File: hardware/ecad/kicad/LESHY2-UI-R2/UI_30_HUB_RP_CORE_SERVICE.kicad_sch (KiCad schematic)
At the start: 47 parts, among them J10 Samtec FTSH-105-01-L-DV-K-P-TR, J11 GCT USB4105-GF-A, SW20 Alps Alpine SKRTLAE010, SW21 Alps Alpine SKRTLAE010, U28 SC1512-A4, U29 Texas Instruments TPD4E05U06D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, U30 Texas Instruments TPD2EUSB30A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, U31 onsemi FSUSB42MUX, Y1 Abracon ABM8-272-T3

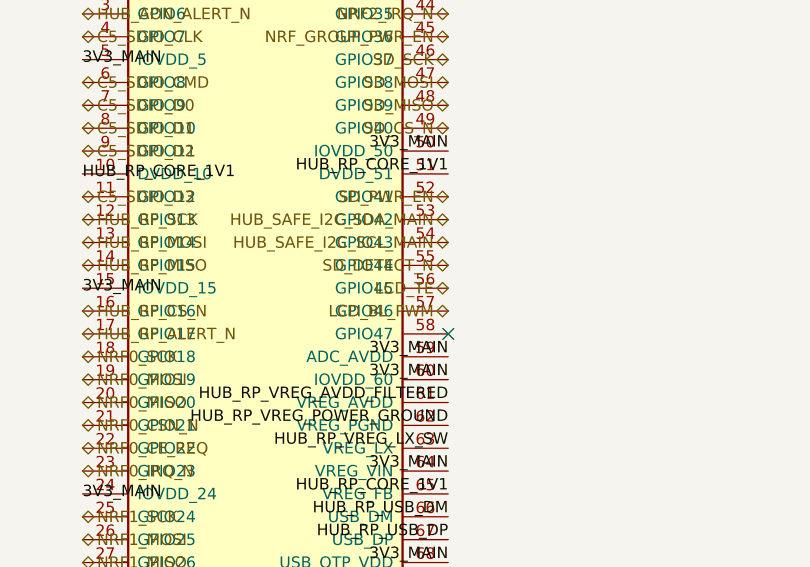
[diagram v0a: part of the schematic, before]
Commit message: Mount display through direct UI-board ZIF
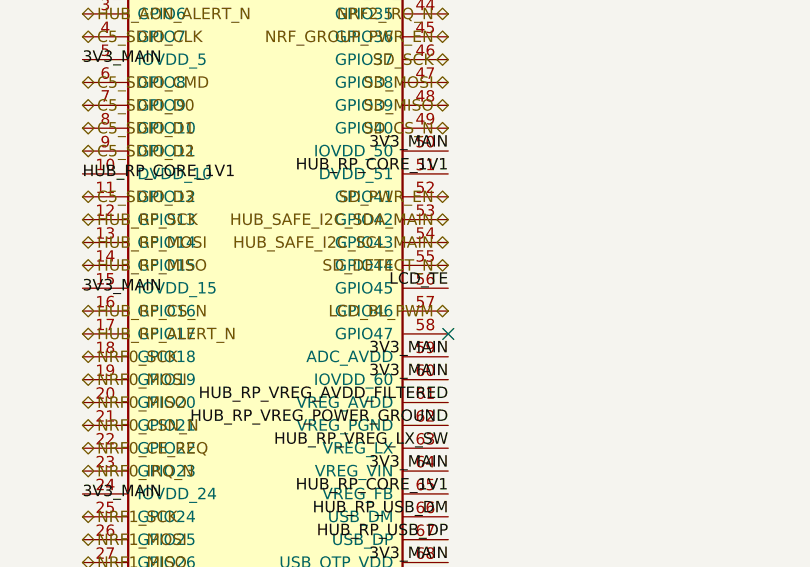
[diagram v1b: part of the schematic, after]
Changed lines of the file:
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@@
 		(effects (font (size 1.27 1.27)) (justify right bottom))
 	)
-	(hierarchical_label "LCD_TE"
-		(shape bidirectional)
+	(label "LCD_TE"
 		(at 624.84 190.50 180)
 		(effects (font (size 1.27 1.27)) (justify right bottom))
